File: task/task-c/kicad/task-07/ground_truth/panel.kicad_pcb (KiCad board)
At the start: 2 copper layers, 143 x 100 mm, 22 parts

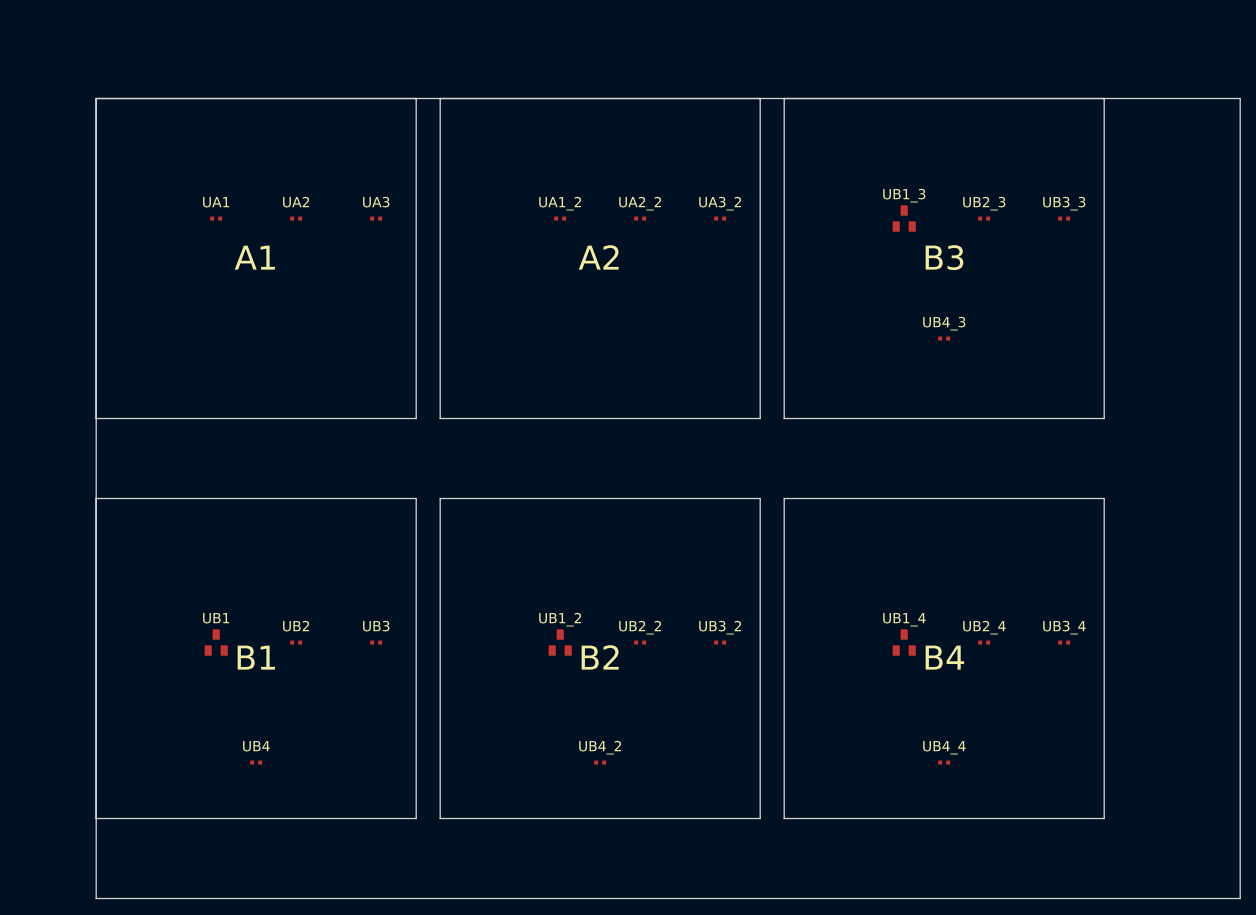
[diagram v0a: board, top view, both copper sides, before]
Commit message: Sync harder Blender Eagle KiCad tasks to final
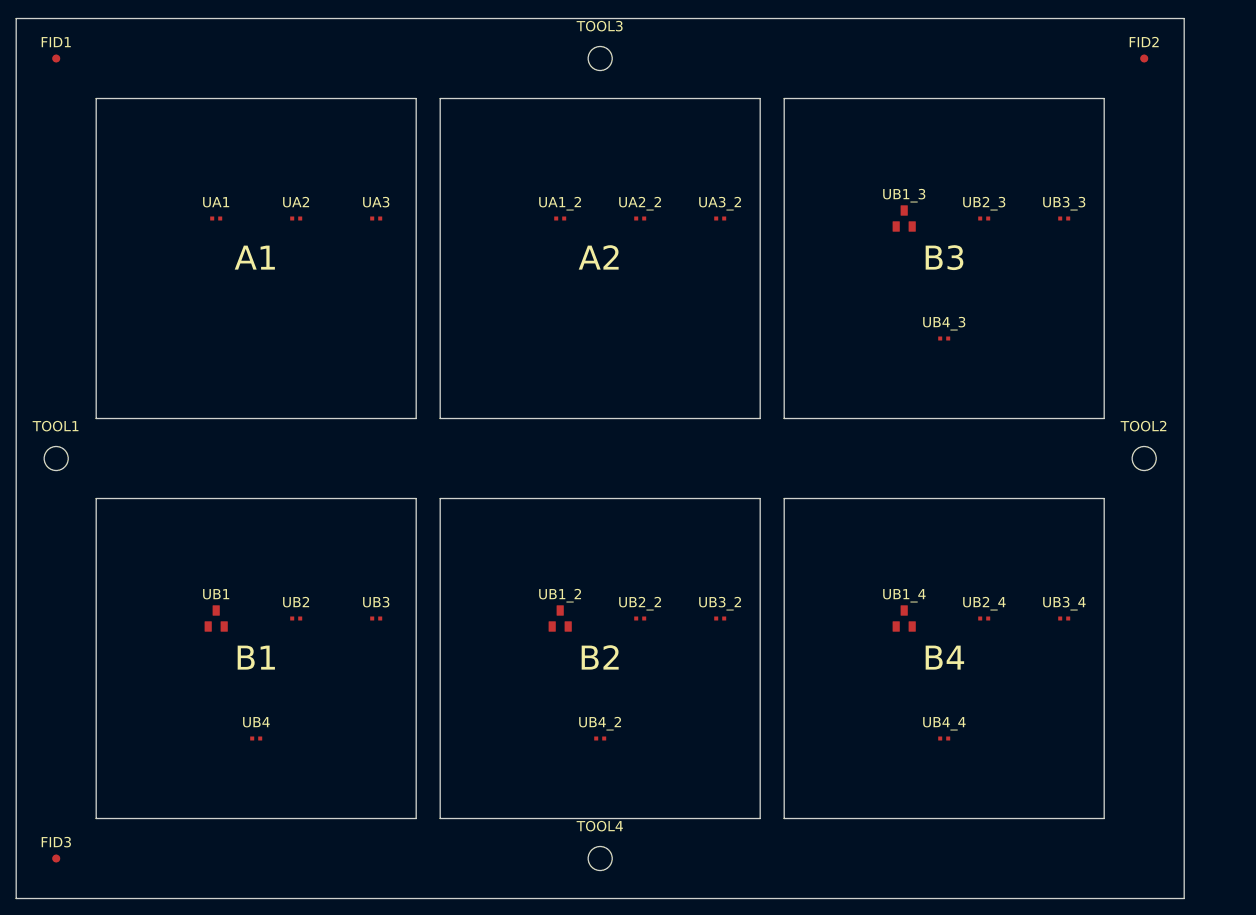
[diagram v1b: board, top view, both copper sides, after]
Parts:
- added FID1: Fiducial, Fiducial:Fiducial_1mm_Mask2mm, F.Cu at (5.00, 5.00)
- added FID2: Fiducial, Fiducial:Fiducial_1mm_Mask2mm, F.Cu at (141.0, 5.00)
- added FID3: Fiducial, Fiducial:Fiducial_1mm_Mask2mm, F.Cu at (5.00, 105.0)
- added TOOL1: NPTH 3.0mm, MountingHole:MountingHole_3.0mm, F.Cu at (5.00, 55.0)
- added TOOL2: NPTH 3.0mm, MountingHole:MountingHole_3.0mm, F.Cu at (141.0, 55.0)
- added TOOL3: NPTH 3.0mm, MountingHole:MountingHole_3.0mm, F.Cu at (73.0, 5.00)
- added TOOL4: NPTH 3.0mm, MountingHole:MountingHole_3.0mm, F.Cu at (73.0, 105.0)
- moved UB1 3.00 mm to (25.0, 75.0)
- moved UB1_2 3.00 mm to (68.0, 75.0)
- moved UB1_4 3.00 mm to (111.0, 75.0)
- moved UB2 3.00 mm to (35.0, 75.0)
- moved UB2_2 3.00 mm to (78.0, 75.0)
- moved UB2_4 3.00 mm to (121.0, 75.0)
- moved UB3 3.00 mm to (45.0, 75.0)
- moved UB3_2 3.00 mm to (88.0, 75.0)
- moved UB3_4 3.00 mm to (131.0, 75.0)
- moved UB4 3.00 mm to (30.0, 90.0)
- moved UB4_2 3.00 mm to (73.0, 90.0)
- moved UB4_4 3.00 mm to (116.0, 90.0)
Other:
- board size 143 x 100 mm -> 146 x 110 mm
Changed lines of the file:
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@@
     (37 "F.Silkscreen" user "F.Silkscreen")
     (39 "F.Fab" user "F.Fab")
+    (40 "Dwgs.User" user "User.Drawings")
     (44 "Edge.Cuts" user "Edge.Cuts")
   )
@@
   )
   (footprint "Package_TO_SOT_SMD:SOT-23"
-    (layer "F.Cu") (uuid "pan-b1-q1") (at 25 78)
+    (layer "F.Cu") (uuid "pan-b1-q1") (at 25 75)
     (property "Reference" "UB1" (at 0 -3 0) (layer "F.Silkscreen") (uuid "pan-b1-q1-ref"))
     (property "Value" "2N3904" (at 0 3 0) (layer "F.Fab") (uuid "pan-b1-q1-val"))
@@
   )
   (footprint "Resistor_SMD:R_0402_1005Metric"
-    (layer "F.Cu") (uuid "pan-b1-r1") (at 35 78)
+    (layer "F.Cu") (uuid "pan-b1-r1") (at 35 75)
     (property "Reference" "UB2" (at 0 -2 0) (layer "F.Silkscreen") (uuid "pan-b1-r1-ref"))
     (property "Value" "4.7k" (at 0 2 0) (layer "F.Fab") (uuid "pan-b1-r1-val"))
@@
   )
   (footprint "Resistor_SMD:R_0402_1005Metric"
-    (layer "F.Cu") (uuid "pan-b1-r2") (at 45 78)
+    (layer "F.Cu") (uuid "pan-b1-r2") (at 45 75)
     (property "Reference" "UB3" (at 0 -2 0) (layer "F.Silkscreen") (uuid "pan-b1-r2-ref"))
     (property "Value" "1k" (at 0 2 0) (layer "F.Fab") (uuid "pan-b1-r2-val"))
@@
   )
   (footprint "Capacitor_SMD:C_0402_1005Metric"
-    (layer "F.Cu") (uuid "pan-b1-c1") (at 30 93)
+    (layer "F.Cu") (uuid "pan-b1-c1") (at 30 90)
     (property "Reference" "UB4" (at 0 -2 0) (layer "F.Silkscreen") (uuid "pan-b1-c1-ref"))
     (property "Value" "10nF" (at 0 2 0) (layer "F.Fab") (uuid "pan-b1-c1-val"))
@@
   )
   (footprint "Package_TO_SOT_SMD:SOT-23"
-    (layer "F.Cu") (uuid "pan-b2-q1") (at 68 78)
+    (layer "F.Cu") (uuid "pan-b2-q1") (at 68 75)
     (property "Reference" "UB1_2" (at 0 -3 0) (layer "F.Silkscreen") (uuid "pan-b2-q1-ref"))
     (property "Value" "2N3904" (at 0 3 0) (layer "F.Fab") (uuid "pan-b2-q1-val"))
@@
   )
   (footprint "Resistor_SMD:R_0402_1005Metric"
-    (layer "F.Cu") (uuid "pan-b2-r1") (at 78 78)
+    (layer "F.Cu") (uuid "pan-b2-r1") (at 78 75)
     (property "Reference" "UB2_2" (at 0 -2 0) (layer "F.Silkscreen") (uuid "pan-b2-r1-ref"))
     (property "Value" "4.7k" (at 0 2 0) (layer "F.Fab") (uuid "pan-b2-r1-val"))
@@
   )
   (footprint "Resistor_SMD:R_0402_1005Metric"
-    (layer "F.Cu") (uuid "pan-b2-r2") (at 88 78)
+    (layer "F.Cu") (uuid "pan-b2-r2") (at 88 75)
     (property "Reference" "UB3_2" (at 0 -2 0) (layer "F.Silkscreen") (uuid "pan-b2-r2-ref"))
     (property "Value" "1k" (at 0 2 0) (layer "F.Fab") (uuid "pan-b2-r2-val"))
@@
   )
   (footprint "Capacitor_SMD:C_0402_1005Metric"
-    (layer "F.Cu") (uuid "pan-b2-c1") (at 73 93)
+    (layer "F.Cu") (uuid "pan-b2-c1") (at 73 90)
     (property "Reference" "UB4_2" (at 0 -2 0) (layer "F.Silkscreen") (uuid "pan-b2-c1-ref"))
     (property "Value" "10nF" (at 0 2 0) (layer "F.Fab") (uuid "pan-b2-c1-val"))
@@
   )
   (footprint "Package_TO_SOT_SMD:SOT-23"
-    (layer "F.Cu") (uuid "pan-b4-q1") (at 111 78)
+    (layer "F.Cu") (uuid "pan-b4-q1") (at 111 75)
     (property "Reference" "UB1_4" (at 0 -3 0) (layer "F.Silkscreen") (uuid "pan-b4-q1-ref"))
     (property "Value" "2N3904" (at 0 3 0) (layer "F.Fab") (uuid "pan-b4-q1-val"))
@@
   )
   (footprint "Resistor_SMD:R_0402_1005Metric"
-    (layer "F.Cu") (uuid "pan-b4-r1") (at 121 78)
+    (layer "F.Cu") (uuid "pan-b4-r1") (at 121 75)
     (property "Reference" "UB2_4" (at 0 -2 0) (layer "F.Silkscreen") (uuid "pan-b4-r1-ref"))
     (property "Value" "4.7k" (at 0 2 0) (layer "F.Fab") (uuid "pan-b4-r1-val"))
@@
   )
   (footprint "Resistor_SMD:R_0402_1005Metric"
-    (layer "F.Cu") (uuid "pan-b4-r2") (at 131 78)
+    (layer "F.Cu") (uuid "pan-b4-r2") (at 131 75)
     (property "Reference" "UB3_4" (at 0 -2 0) (layer "F.Silkscreen") (uuid "pan-b4-r2-ref"))
     (property "Value" "1k" (at 0 2 0) (layer "F.Fab") (uuid "pan-b4-r2-val"))
@@
   )
   (footprint "Capacitor_SMD:C_0402_1005Metric"
-    (layer "F.Cu") (uuid "pan-b4-c1") (at 116 93)
+    (layer "F.Cu") (uuid "pan-b4-c1") (at 116 90)
     (property "Reference" "UB4_4" (at 0 -2 0) (layer "F.Silkscreen") (uuid "pan-b4-c1-ref"))
     (property "Value" "10nF" (at 0 2 0) (layer "F.Fab") (uuid "pan-b4-c1-val"))
@@
     (pad "2" smd rect (at 0.5 0) (size 0.5 0.5) (layers "F.Cu" "F.Paste" "F.Mask") (net 2 "GND") (uuid "pan-b4-c1-p2"))
   )
-  (gr_line (start 10 10) (end 153 10) (layer "Edge.Cuts") (width 0.05) (uuid "pan-outer-top"))
-  (gr_line (start 153 10) (end 153 110) (layer "Edge.Cuts") (width 0.05) (uuid "pan-outer-right"))
-  (gr_line (start 153 110) (end 10 110) (layer "Edge.Cuts") (width 0.05) (uuid "pan-outer-bottom"))
-  (gr_line (start 10 110) (end 10 10) (layer "Edge.Cuts") (width 0.05) (uuid "pan-outer-left"))
+  (gr_line (start 0 0) (end 146 0) (layer "Edge.Cuts") (width 0.05) (uuid "pan-outer-top"))
+  (gr_line (start 146 0) (end 146 110) (layer "Edge.Cuts") (width 0.05) (uuid "pan-outer-right"))
+  (gr_line (start 146 110) (end 0 110) (layer "Edge.Cuts") (width 0.05) (uuid "pan-outer-bottom"))
+  (gr_line (start 0 110) (end 0 0) (layer "Edge.Cuts") (width 0.05) (uuid "pan-outer-left"))
   (gr_line (start 10 10) (end 50 10) (layer "Edge.Cuts") (width 0.05) (uuid "a1-top"))
   (gr_line (start 50 10) (end 50 50) (layer "Edge.Cuts") (width 0.05) (uuid "a1-right"))
@@
   (gr_text "B4" (at 116 80) (layer "F.Silkscreen") (uuid "lbl-b4")
     (effects (font (size 3 3) (thickness 0.5))))
+  (gr_line (start 50 10) (end 50 100) (layer "Dwgs.User") (width 0.12) (uuid "vscore-x50"))
+  (gr_line (start 93 10) (end 93 100) (layer "Dwgs.User") (width 0.12) (uuid "vscore-x93"))
+  (gr_line (start 10 55) (end 136 55) (layer "Dwgs.User") (width 0.12) (uuid "vscore-y55"))
+  (footprint "Fiducial:Fiducial_1mm_Mask2mm" (layer "F.Cu") (uuid "fid1") (at 5 5)
+    (property "Reference" "FID1" (at 0 -2 0) (layer "F.Silkscreen") (uuid "fid1-ref"))
+    (property "Value" "Fiducial" (at 0 2 0) (layer "F.Fab") (uuid "fid1-val"))
+    (pad "1" smd circle (at 0 0) (size 1 1) (layers "F.Cu" "F.Mask") (uuid "fid1-pad"))
+  )
+  (footprint "Fiducial:Fiducial_1mm_Mask2mm" (layer "F.Cu") (uuid "fid2") (at 141 5)
+    (property "Reference" "FID2" (at 0 -2 0) (layer "F.Silkscreen") (uuid "fid2-ref"))
+    (property "Value" "Fiducial" (at 0 2 0) (layer "F.Fab") (uuid "fid2-val"))
+    (pad "1" smd circle (at 0 0) (size 1 1) (layers "F.Cu" "F.Mask") (uuid "fid2-pad"))
+  )
+  (footprint "Fiducial:Fiducial_1mm_Mask2mm" (layer "F.Cu") (uuid "fid3") (at 5 105)
+    (property "Reference" "FID3" (at 0 -2 0) (layer "F.Silkscreen") (uuid "fid3-ref"))
+    (property "Value" "Fiducial" (at 0 2 0) (layer "F.Fab") (uuid "fid3-val"))
+    (pad "1" smd circle (at 0 0) (size 1 1) (layers "F.Cu" "F.Mask") (uuid "fid3-pad"))
+  )
+  (footprint "MountingHole:MountingHole_3.0mm" (layer "F.Cu") (uuid "tool1") (at 5 55)
+    (property "Reference" "TOOL1" (at 0 -4 0) (layer "F.Silkscreen") (uuid "tool1-ref"))
+    (property "Value" "NPTH 3.0mm" (at 0 4 0) (layer "F.Fab") (uuid "tool1-val"))
+    (pad "" np_thru_hole circle (at 0 0) (size 3 3) (drill 3) (layers "*.Cu" "*.Mask") (uuid "tool1-pad"))
+  )
+  (footprint "MountingHole:MountingHole_3.0mm" (layer "F.Cu") (uuid "tool2") (at 141 55)
+    (property "Reference" "TOOL2" (at 0 -4 0) (layer "F.Silkscreen") (uuid "tool2-ref"))
+    (property "Value" "NPTH 3.0mm" (at 0 4 0) (layer "F.Fab") (uuid "tool2-val"))
+    (pad "" np_thru_hole circle (at 0 0) (size 3 3) (drill 3) (layers "*.Cu" "*.Mask") (uuid "tool2-pad"))
+  )
+  (footprint "MountingHole:MountingHole_3.0mm" (layer "F.Cu") (uuid "tool3") (at 73 5)
+    (property "Reference" "TOOL3" (at 0 -4 0) (layer "F.Silkscreen") (uuid "tool3-ref"))
+    (property "Value" "NPTH 3.0mm" (at 0 4 0) (layer "F.Fab") (uuid "tool3-val"))
+    (pad "" np_thru_hole circle (at 0 0) (size 3 3) (drill 3) (layers "*.Cu" "*.Mask") (uuid "tool3-pad"))
+  )
+  (footprint "MountingHole:MountingHole_3.0mm" (layer "F.Cu") (uuid "tool4") (at 73 105)
+    (property "Reference" "TOOL4" (at 0 -4 0) (layer "F.Silkscreen") (uuid "tool4-ref"))
+    (property "Value" "NPTH 3.0mm" (at 0 4 0) (layer "F.Fab") (uuid "tool4-val"))
+    (pad "" np_thru_hole circle (at 0 0) (size 3 3) (drill 3) (layers "*.Cu" "*.Mask") (uuid "tool4-pad"))
+  )
 )
